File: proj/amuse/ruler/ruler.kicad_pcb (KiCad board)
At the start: 2 copper layers, 175 x 15 mm, 2 parts

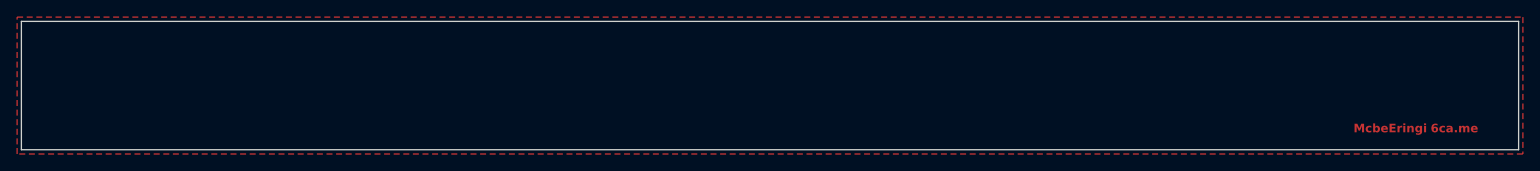
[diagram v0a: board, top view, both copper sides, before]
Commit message: -
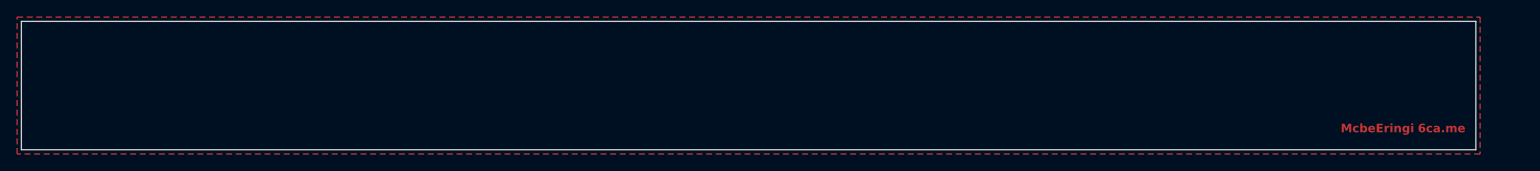
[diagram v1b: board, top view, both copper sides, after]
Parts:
- moved ? 1.50 mm to (263.4, 104.9)
- moved ? 1.50 mm to (258.5, 107.5)
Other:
- board size 175 x 15 mm -> 170 x 15 mm
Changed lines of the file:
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@@
 	(footprint "QRCODE"
 		(layer "F.Cu")
-		(at 264.875 104.875)
+		(at 263.375 104.875)
 		(property "Reference" ""
 			(at 0 0 0)
@@
 	(footprint "Library:mcbeeringi_icon_10mm"
 		(layer "F.Cu")
-		(at 260 107.5)
+		(at 258.5 107.5)
 		(property "Reference" ""
 			(at 0 0 0)
@@
 	)
 	(gr_line
-		(start 275 115)
-		(end 275 100)
+		(start 270 115)
+		(end 270 100)
 		(stroke
 			(width 0.05)
@@
 	)
 	(gr_line
-		(start 275 115)
+		(start 270 115)
 		(end 100 115)
 		(stroke
@@
 	(gr_line
 		(start 100 100)
-		(end 275 100)
+		(end 270 100)
 		(stroke
 			(width 0.05)
@@
 	)
 	(gr_text "McbeEringi"
-		(at 260 112.5 0)
+		(at 258.5 112.5 0)
 		(layer "F.Cu" knockout)
 		(effects
@@
 	)
 	(gr_text "6ca.me"
-		(at 267.5 112.5 0)
+		(at 266 112.5 0)
 		(layer "F.Cu" knockout)
 		(effects
@@
 		(polygon
 			(pts
-				(xy 99.5 99.5) (xy 275.5 99.5) (xy 275.5 115.5) (xy 99.5 115.5)
+				(xy 99.5 99.5) (xy 270.5 99.5) (xy 270.5 115.5) (xy 99.5 115.5)
 			)
 		)
@@
 		(polygon
 			(pts
-				(xy 99.5 99.5) (xy 275.5 99.5) (xy 275.5 115.5) (xy 99.5 115.5)
+				(xy 99.5 99.5) (xy 270.5 99.5) (xy 270.5 115.5) (xy 99.5 115.5)
 			)
 		)
